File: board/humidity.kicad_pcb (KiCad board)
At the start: 2 copper layers, 22 x 88 mm, 26 parts, among them IC101 ATTINY13A-SS, P101 TST, P102 TST, P103 TST, P104 TST, P105 CONN_2, Q101 PNP

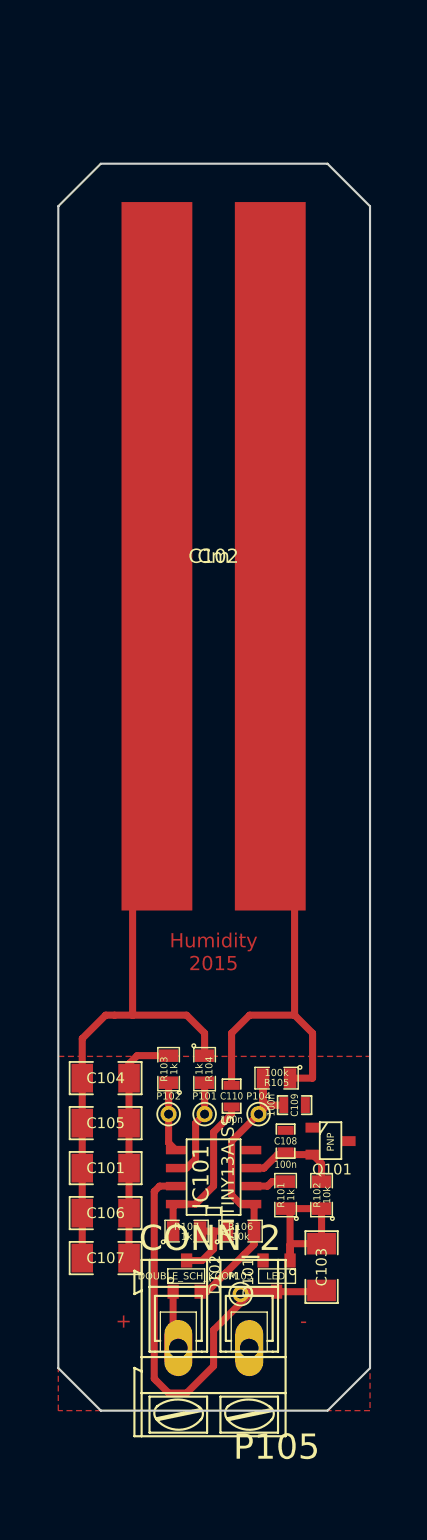
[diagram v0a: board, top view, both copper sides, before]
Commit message: Initial Revision of Controller schematic
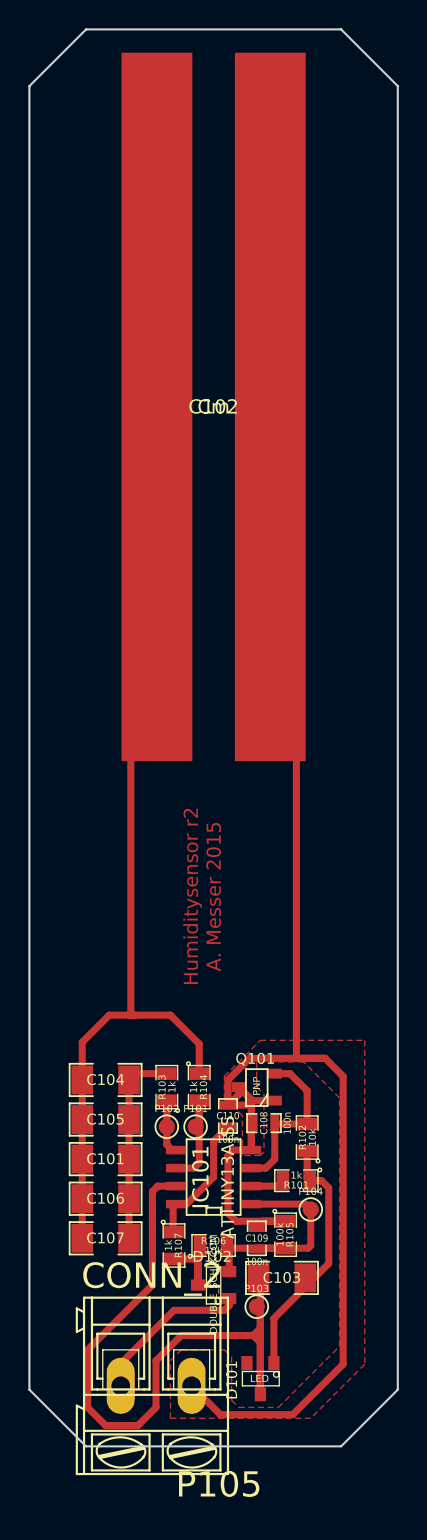
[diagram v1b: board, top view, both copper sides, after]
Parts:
- moved R105 11.1 mm to (66.0, 100.6), turned to 270 degrees
- moved C102 10.5 mm to (61.0, 42.2)
- moved C109 9.77 mm to (64.0, 100.8), turned to 90 degrees
- moved P104 7.67 mm to (67.8, 98.8)
- moved D101 7.33 mm to (64.3, 110.7)
- moved Q101 6.45 mm to (64.0, 90.2), turned to 90 degrees
- moved P105 4.86 mm to (56.9, 111.3)
- moved R102 4.19 mm to (67.6, 93.7)
- moved C103 2.90 mm to (65.8, 103.6), turned to 180 degrees
- moved R106 2.16 mm to (61.0, 101.3)
- moved D102 2.01 mm to (61.0, 104.1), turned to 90 degrees
- moved C108 1.98 mm to (64.5, 92.7), turned to 180 degrees
- moved P103 1.45 mm to (64.0, 105.7)
- moved C110 1.42 mm to (62.0, 92.2)
- moved C107 1.40 mm to (53.3, 100.8)
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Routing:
- net GND: track 48.3 -> 121.6 mm
- net N-0000012: track 34.9 -> 59.0 mm
- net N-0000014: track 60.0 -> 70.1 mm
- net N-000006: track 4.13 -> 11.4 mm
- net N-000007: track 23.0 -> 16.9 mm
- net N-000001: track 12.2 -> 18.1 mm
- net N-000003: track 6.88 -> 11.9 mm
- net N-0000013: track 16.1 -> 14.0 mm
- net N-000008: track 11.3 -> 9.42 mm
- net N-0000010: track 4.97 -> 3.90 mm
- net VCC: track 5.41 -> 6.25 mm
- net N-0000011: track 7.32 -> 8.14 mm
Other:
- board size 22 x 88 mm -> 26 x 100 mm
- board text added: "Humiditysensor r2 A. Messer 2015"
- board text removed: "+"
- board text removed: "-"
- board text removed: "Humidity 2015"

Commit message: Fix nterchanges RESET and CS pin of display
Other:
- net class Default: clearance 0.254 -> 0.25; trace_width 0.254 -> 0.3
- rule trace_clearance: 0.254 -> 0.25
- rule trace_min: 0.254 -> 0.3
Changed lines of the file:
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@@
     (links 43)
     (no_connects 0)
-    (area 31.58131 24.924999 90.33869 116.75745)
+    (area 31.58531 15.444999 90.33469 119.42045)
     (thickness 1.6)
     (drawings 18)
@@
   )
   (setup
-    (last_trace_width 0.5)
+    (last_trace_width 0.3)
     (user_trace_width 0.5)
     (user_trace_width 0.7)
-    (trace_clearance 0.254)
+    (trace_clearance 0.25)
     (zone_clearance 0.5)
     (zone_45_only no)
-    (trace_min 0.254)
+    (trace_min 0.3)
     (segment_width 0.2)
     (edge_width 0.15)
@@
       (padsonsilk false)
       (subtractmaskfromsilk false)
-      (outputformat 5)
+      (outputformat 2)
       (mirror false)
       (drillshape 1)
@@
   (net 13 VCC)
   (net_class Default "Dies ist die voreingestellte Netzklasse."
-    (clearance 0.254)
-    (trace_width 0.254)
+    (clearance 0.25)
+    (trace_width 0.3)
     (via_dia 0.889)
     (via_drill 0.635)
@@
   (segment (start 59.944 95.504) (end 59.944 91.1225) (width 0.5) (layer F.Cu) (net 4))
   (segment (start 59.563 95.885) (end 59.944 95.504) (width 0.5) (layer F.Cu) (net 4))
-  (segment (start 64.008 105.664) (end 64.262 105.918) (width 0.5) (layer F.Cu) (net 5) (status C00000))
-  (segment (start 64.262 105.918) (end 64.262 111.84382) (width 0.5) (layer F.Cu) (net 5) (status C00000))
+  (segment (start 64.008 105.664) (end 64.262 105.918) (width 0.5) (layer F.Cu) (net 5))
+  (segment (start 64.262 105.918) (end 64.262 111.84382) (width 0.5) (layer F.Cu) (net 5))
   (segment (start 52.07 112.776) (end 53.34 114.046) (width 0.5) (layer F.Cu) (net 5))
   (segment (start 55.626 114.046) (end 56.896 112.776) (width 0.5) (layer F.Cu) (net 5))
